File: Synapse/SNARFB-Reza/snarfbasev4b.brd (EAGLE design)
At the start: 90 x 56 mm, 54 parts, among them J1 AVR_SPI_PRG_6PTH, J2 POWER_JACKPTH, U1 PCF2129ASO20, U2 lm75adp, U3 TSL2561_DFN, U4 ATMEGA32U4-AU, U5 24LC256T-I/SN, U6 PCA9541SO16-2, U8 MAX3232EIDWR, X1 USBSMD

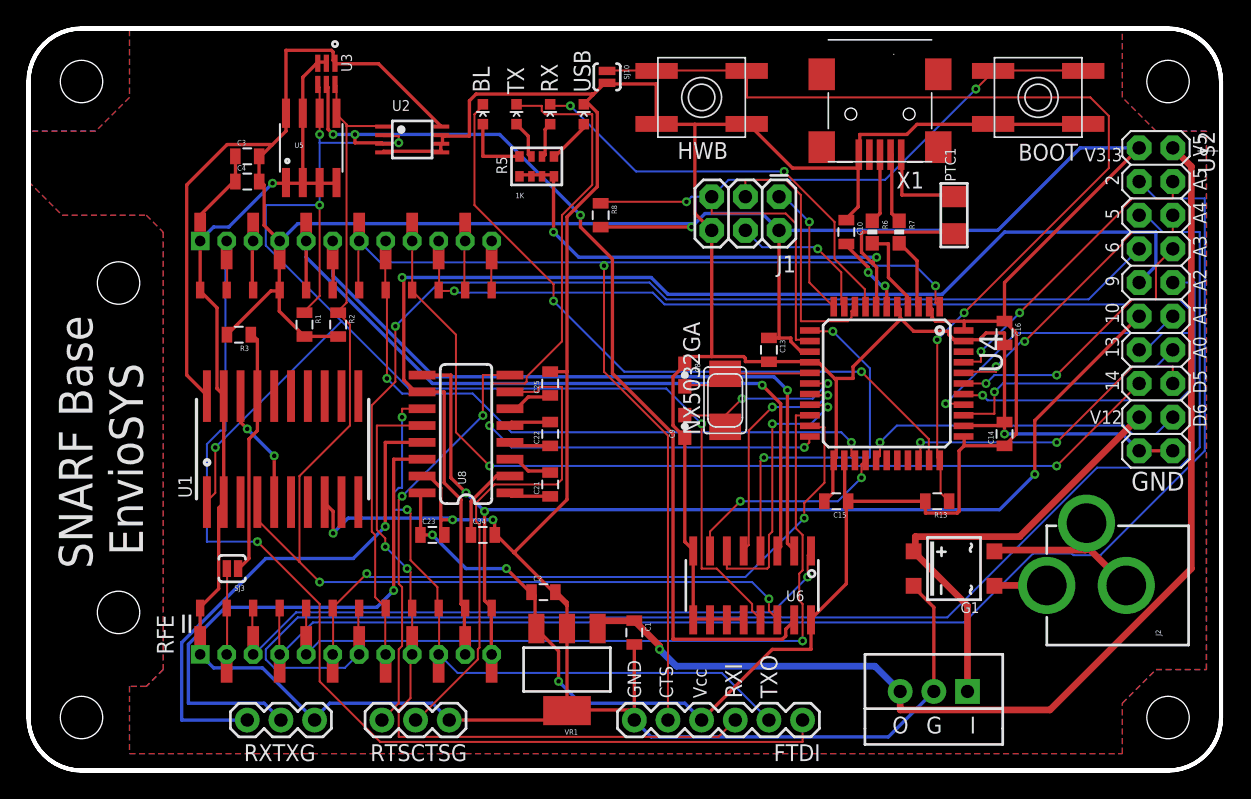
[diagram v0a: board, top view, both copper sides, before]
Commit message: sync
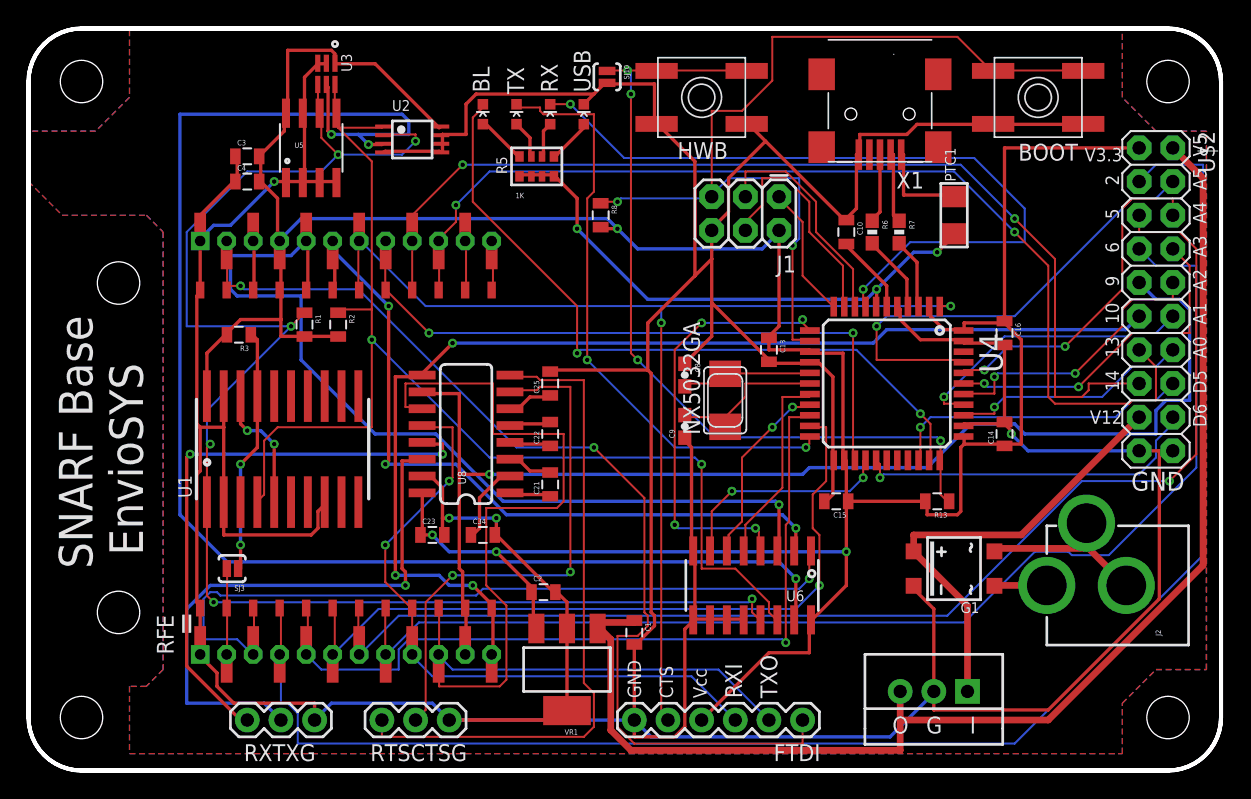
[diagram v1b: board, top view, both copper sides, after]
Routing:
- net GND: track 395.5 -> 451.6 mm, vias 5 -> 4
- net !TLINT: track 72.9 -> 112.3 mm
- net TXO: track 50.8 -> 81.8 mm, vias 2 -> 0
- net ARXLED: track 32.6 -> 56.7 mm
- net VCC3: track 270.8 -> 246.8 mm
- net RTS1: track 31.4 -> 49.8 mm, vias 2 -> 0
- net GPIO2_PINHD: track 105.7 -> 121.6 mm
- net GPIO5_PINHD: track 110.3 -> 94.6 mm, vias 0 -> 1
- net ATXLED: track 59.9 -> 45.4 mm
- net PF0-A5: track 22.7 -> 36.0 mm, vias 2 -> 1
- net VCC5: track 85.9 -> 98.5 mm, vias 1 -> 0
- net HWB: track 75.3 -> 63.2 mm, vias 2 -> 4
- net RST: track 58.5 -> 69.6 mm
- net GPIO13_PINHD: track 67.5 -> 78.4 mm, vias 1 -> 2
- net SCL0: track 57.8 -> 68.4 mm
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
